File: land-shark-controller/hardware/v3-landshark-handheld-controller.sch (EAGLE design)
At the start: 10 parts

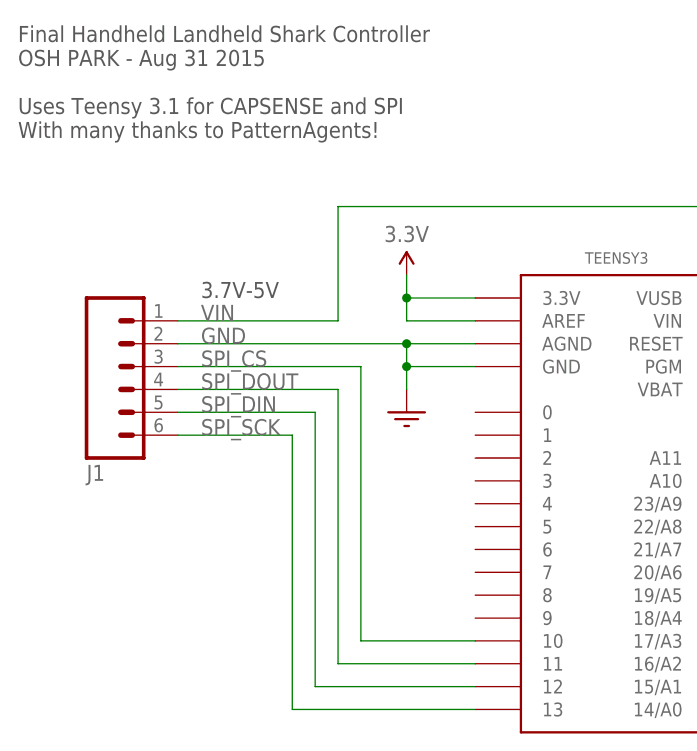
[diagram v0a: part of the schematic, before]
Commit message: Added v3 gerbers, final board. Added 7-pin breakout as per feeeeture creeeeep. Use the gerbers, I took some silk off the top layer.
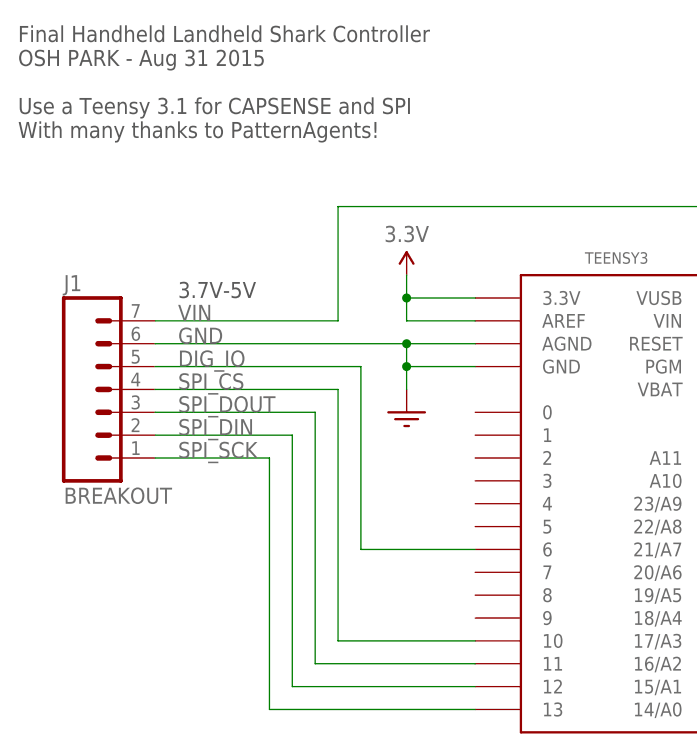
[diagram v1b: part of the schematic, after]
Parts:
- J1: value (none) -> BREAKOUT; device SparkFun-Connectors:M06LOCK_LONGPADS -> SparkFun-Connectors:M07LOCK_LONGPADS
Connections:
- new net DIG_IO: J1.5, TEENSY3.6
- net GND: now also J1.6; no longer J1.2
- net SPI_CS: now also J1.4; no longer J1.3
- net SPI_DIN: now also J1.2; no longer J1.5
- net SPI_DOUT: now also J1.3; no longer J1.4
- net SPI_SCK: now also J1.1; no longer J1.6
- net VIN: now also J1.7; no longer J1.1
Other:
- note added: "Final Handheld Landheld Shark Controller OSH PARK - Aug 31 2015 Use a Teensy 3.1 for CAPSENSE and SPI With many thanks to PatternAgents!"
- note removed: "Final Handheld Landheld Shark Controller OSH PARK - Aug 31 2015 Uses Teensy 3.1 for CAPSENSE and SPI With many thanks to PatternAgents!"
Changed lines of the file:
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@@
 <part name="H1" library="holes" deviceset="MOUNT-HOLE" device="4.1" value="MOUNT-HOLE4.1"/>
 <part name="H2" library="holes" deviceset="MOUNT-HOLE" device="4.1" value="MOUNT-HOLE4.1"/>
-<part name="J1" library="SparkFun-Connectors" deviceset="M06" device="LOCK_LONGPADS"/>
+<part name="J1" library="SparkFun-Connectors" deviceset="M07" device="LOCK_LONGPADS" value="BREAKOUT"/>
 </parts>
 <sheets>
@@
 <text x="7.62" y="78.74" size="1.778" layer="97">Final Handheld Landheld Shark Controller
 OSH PARK - Aug 31 2015
-Uses Teensy 3.1 for CAPSENSE and SPI
+Use a Teensy 3.1 for CAPSENSE and SPI
 With many thanks to PatternAgents!</text>
-<text x="27.94" y="60.96" size="1.778" layer="97">3.7V-5V</text>
+<text x="25.4" y="60.96" size="1.778" layer="97">3.7V-5V</text>
 <text x="110.49" y="82.55" size="1.778" layer="97">4.1MM MOUNTING HOLES</text>
 <wire x1="109.22" y1="81.28" x2="109.22" y2="63.5" width="0.1524" layer="97" style="longdash"/>
@@
 <instance part="H1" gate="G$1" x="114.3" y="76.2"/>
 <instance part="H2" gate="G$1" x="114.3" y="68.58"/>
-<instance part="J1" gate="G$1" x="20.32" y="53.34" rot="MR180"/>
+<instance part="J1" gate="G$1" x="17.78" y="48.26"/>
 </instances>
 <busses>
@@
 <wire x1="50.8" y1="55.88" x2="50.8" y2="53.34" width="0.1524" layer="91"/>
 <junction x="50.8" y="53.34"/>
-<wire x1="25.4" y1="55.88" x2="50.8" y2="55.88" width="0.1524" layer="91"/>
+<wire x1="22.86" y1="55.88" x2="50.8" y2="55.88" width="0.1524" layer="91"/>
 <junction x="50.8" y="55.88"/>
-<label x="27.94" y="55.88" size="1.778" layer="95"/>
-<pinref part="J1" gate="G$1" pin="2"/>
+<label x="25.4" y="55.88" size="1.778" layer="95"/>
+<pinref part="J1" gate="G$1" pin="6"/>
 </segment>
 </net>
@@
 <net name="SPI_SCK" class="0">
 <segment>
-<wire x1="25.4" y1="45.72" x2="38.1" y2="45.72" width="0.1524" layer="91"/>
-<wire x1="38.1" y1="45.72" x2="38.1" y2="15.24" width="0.1524" layer="91"/>
+<wire x1="22.86" y1="43.18" x2="35.56" y2="43.18" width="0.1524" layer="91"/>
+<wire x1="35.56" y1="43.18" x2="35.56" y2="15.24" width="0.1524" layer="91"/>
 <pinref part="TEENSY3" gate="G$1" pin="13"/>
-<wire x1="38.1" y1="15.24" x2="58.42" y2="15.24" width="0.1524" layer="91"/>
-<label x="27.94" y="45.72" size="1.778" layer="95"/>
-<pinref part="J1" gate="G$1" pin="6"/>
+<wire x1="35.56" y1="15.24" x2="58.42" y2="15.24" width="0.1524" layer="91"/>
+<label x="25.4" y="43.18" size="1.778" layer="95"/>
+<pinref part="J1" gate="G$1" pin="1"/>
 </segment>
 </net>
@@
 <segment>
 <pinref part="TEENSY3" gate="G$1" pin="12"/>
-<wire x1="58.42" y1="17.78" x2="40.64" y2="17.78" width="0.1524" layer="91"/>
-<wire x1="40.64" y1="17.78" x2="40.64" y2="48.26" width="0.1524" layer="91"/>
-<wire x1="40.64" y1="48.26" x2="25.4" y2="48.26" width="0.1524" layer="91"/>
-<label x="27.94" y="48.26" size="1.778" layer="95"/>
-<pinref part="J1" gate="G$1" pin="5"/>
+<wire x1="58.42" y1="17.78" x2="38.1" y2="17.78" width="0.1524" layer="91"/>
+<wire x1="38.1" y1="17.78" x2="38.1" y2="45.72" width="0.1524" layer="91"/>
+<wire x1="38.1" y1="45.72" x2="22.86" y2="45.72" width="0.1524" layer="91"/>
+<label x="25.4" y="45.72" size="1.778" layer="95"/>
+<pinref part="J1" gate="G$1" pin="2"/>
 </segment>
 </net>
 <net name="SPI_DOUT" class="0">
 <segment>
-<wire x1="25.4" y1="50.8" x2="43.18" y2="50.8" width="0.1524" layer="91"/>
-<wire x1="43.18" y1="50.8" x2="43.18" y2="20.32" width="0.1524" layer="91"/>
+<wire x1="22.86" y1="48.26" x2="40.64" y2="48.26" width="0.1524" layer="91"/>
+<wire x1="40.64" y1="48.26" x2="40.64" y2="20.32" width="0.1524" layer="91"/>
 <pinref part="TEENSY3" gate="G$1" pin="11"/>
-<wire x1="43.18" y1="20.32" x2="58.42" y2="20.32" width="0.1524" layer="91"/>
-<label x="27.94" y="50.8" size="1.778" layer="95"/>
-<pinref part="J1" gate="G$1" pin="4"/>
+<wire x1="40.64" y1="20.32" x2="58.42" y2="20.32" width="0.1524" layer="91"/>
+<label x="25.4" y="48.26" size="1.778" layer="95"/>
+<pinref part="J1" gate="G$1" pin="3"/>
 </segment>
 </net>
@@
 <segment>
 <pinref part="TEENSY3" gate="G$1" pin="10"/>
-<wire x1="58.42" y1="22.86" x2="45.72" y2="22.86" width="0.1524" layer="91"/>
-<wire x1="45.72" y1="22.86" x2="45.72" y2="53.34" width="0.1524" layer="91"/>
-<wire x1="45.72" y1="53.34" x2="25.4" y2="53.34" width="0.1524" layer="91"/>
-<label x="27.94" y="53.34" size="1.778" layer="95"/>
-<pinref part="J1" gate="G$1" pin="3"/>
+<wire x1="58.42" y1="22.86" x2="43.18" y2="22.86" width="0.1524" layer="91"/>
+<wire x1="43.18" y1="22.86" x2="43.18" y2="50.8" width="0.1524" layer="91"/>
+<wire x1="43.18" y1="50.8" x2="22.86" y2="50.8" width="0.1524" layer="91"/>
+<label x="25.4" y="50.8" size="1.778" layer="95"/>
+<pinref part="J1" gate="G$1" pin="4"/>
 </segment>
 </net>
@@
 <wire x1="93.98" y1="71.12" x2="43.18" y2="71.12" width="0.1524" layer="91"/>
 <wire x1="43.18" y1="71.12" x2="43.18" y2="58.42" width="0.1524" layer="91"/>
-<wire x1="43.18" y1="58.42" x2="25.4" y2="58.42" width="0.1524" layer="91"/>
-<label x="27.94" y="58.42" size="1.778" layer="95"/>
-<pinref part="J1" gate="G$1" pin="1"/>
+<wire x1="43.18" y1="58.42" x2="22.86" y2="58.42" width="0.1524" layer="91"/>
+<label x="25.4" y="58.42" size="1.778" layer="95"/>
+<pinref part="J1" gate="G$1" pin="7"/>
 </segment>
 </net>
+<net name="DIG_IO" class="0">
+<segment>
+<pinref part="J1" gate="G$1" pin="5"/>
+<wire x1="22.86" y1="53.34" x2="45.72" y2="53.34" width="0.1524" layer="91"/>
+<wire x1="45.72" y1="53.34" x2="45.72" y2="33.02" width="0.1524" layer="91"/>
+<pinref part="TEENSY3" gate="G$1" pin="6"/>
+<wire x1="45.72" y1="33.02" x2="58.42" y2="33.02" width="0.1524" layer="91"/>
+<label x="25.4" y="53.34" size="1.778" layer="95"/>
+</segment>
+</net>
